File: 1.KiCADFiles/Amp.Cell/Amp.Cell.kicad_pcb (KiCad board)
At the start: 4 copper layers, 20 x 40 mm, 19 parts, among them J4 Conn_01x08, Q1 MMBT3904, Q2 MMBT3906

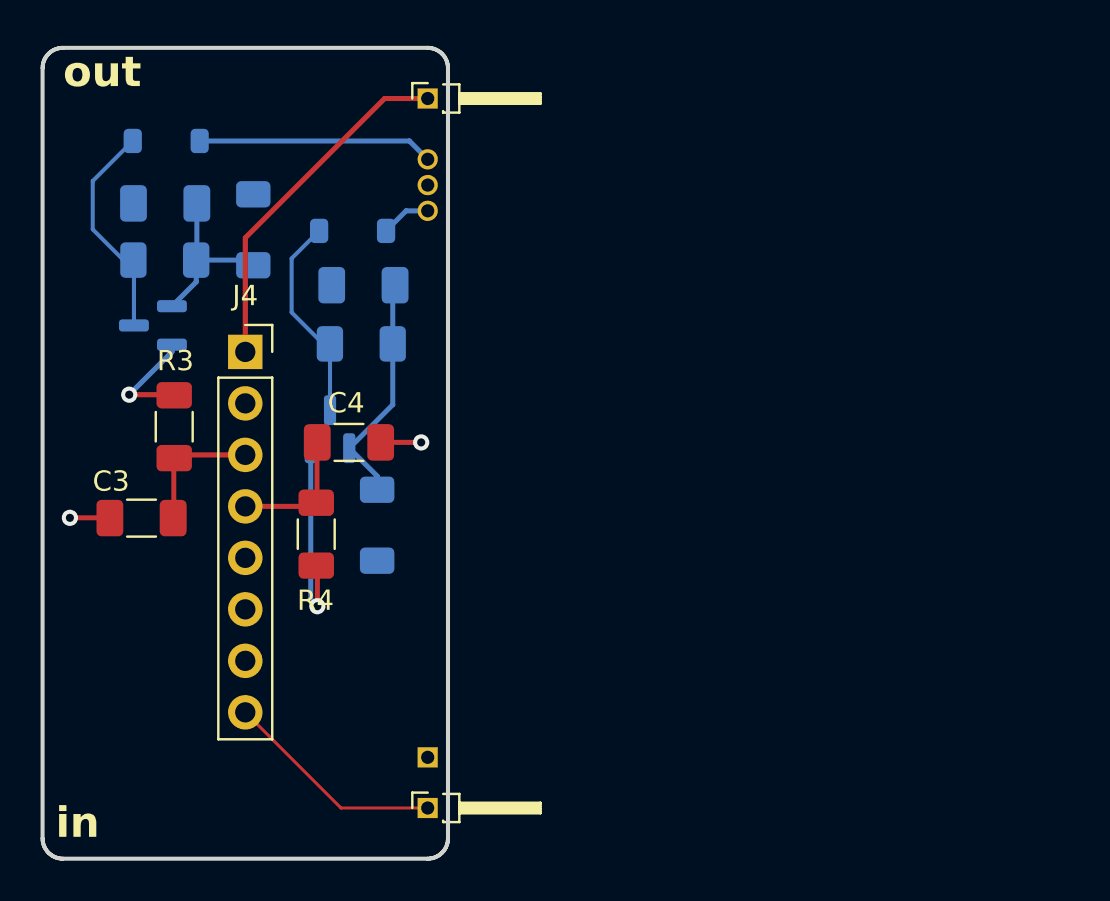
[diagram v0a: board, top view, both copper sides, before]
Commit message: Updated Files
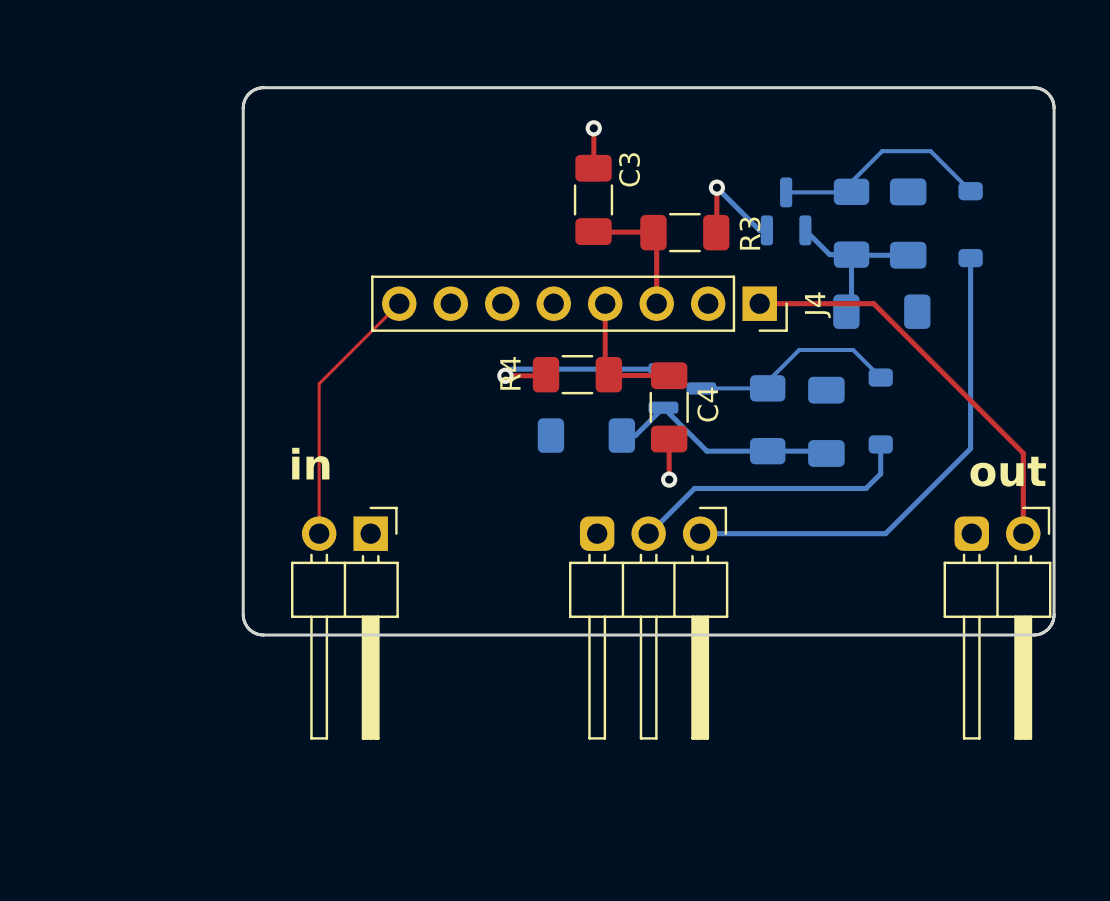
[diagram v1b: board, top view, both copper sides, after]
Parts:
- removed REF** (x3): PinHeader_1x01_P1.27mm_Horizontal, Connector_PinHeader_1.27mm:PinHeader_1x01_P1.27mm_Horizontal
- removed REF**: PinHeader_1x03_P1.27mm_Horizontal, Connector_PinHeader_1.27mm:PinHeader_1x03_P1.27mm_Horizontal
- added REF**10: PinHeader_1x02_P2.54mm_Horizontal, Connector_PinHeader_2.54mm:PinHeader_1x02_P2.54mm_Horizontal, F.Cu at (31.6, 39.4)
- added REF**11: PinHeader_1x03_P2.54mm_Horizontal, Connector_PinHeader_2.54mm:PinHeader_1x03_P2.54mm_Horizontal, F.Cu at (47.8, 39.4)
- added REF**12: PinHeader_1x02_P2.54mm_Horizontal, Connector_PinHeader_2.54mm:PinHeader_1x02_P2.54mm_Horizontal, F.Cu at (63.8, 39.4)
- moved D1 39.9 mm to (61.2, 24.2), turned to -90 degrees
- moved C1 36.7 mm to (58.1, 24.1), turned to 90 degrees
- moved R1 33.9 mm to (55.3, 24.1), turned to -90 degrees
- moved Q1 31.7 mm to (52.1, 23.5), turned to 90 degrees
- moved D3 31.3 mm to (56.8, 28.5), turned to 0 degrees
- moved D2 27.5 mm to (56.7, 33.4), turned to 90 degrees
- moved C3 27.3 mm to (42.6, 23.0), turned to 90 degrees
- moved R3 27.0 mm to (47.1, 24.6), turned to 180 degrees
- moved J4 25.5 mm to (50.8, 28.1), turned to -90 degrees
- moved C2 23.8 mm to (54.1, 33.9), turned to 90 degrees
- moved R2 20.4 mm to (51.2, 33.8), turned to -90 degrees
- moved Q2 17.5 mm to (47.0, 32.3), turned to 0 degrees
- moved C4 15.9 mm to (46.3, 33.2), turned to -90 degrees
- moved R4 15.1 mm to (41.8, 31.6), turned to 0 degrees
- moved D4 11.2 mm to (42.2, 34.6), turned to 0 degrees
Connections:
- D1 pad 2: (no net) -> +
- D2 pad 1: (no net) -> -
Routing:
- net +: track 0.00 -> 24.5 mm
- net -: track 0.00 -> 14.3 mm
- net (no net): track 14.3 -> 0.00 mm
- net Net-(J2-In): track 17.5 -> 20.0 mm
- net Net-(J3-In): track 11.0 -> 13.0 mm
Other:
- board size 20 x 40 mm -> 40 x 27 mm
